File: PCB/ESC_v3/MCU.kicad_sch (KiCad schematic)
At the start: 48 parts, among them J10 Conn_01x01_Pin, J3 Conn_01x01_Pin, J4 Conn_01x01_Pin, J5 Conn_01x01_Pin, J6 Conn_01x01_Pin, J7 Conn_01x01_Pin, J8 Conn_01x01_Pin, J9 Conn_01x01_Pin, U3 STM32G474CETx, Y2 24MHz

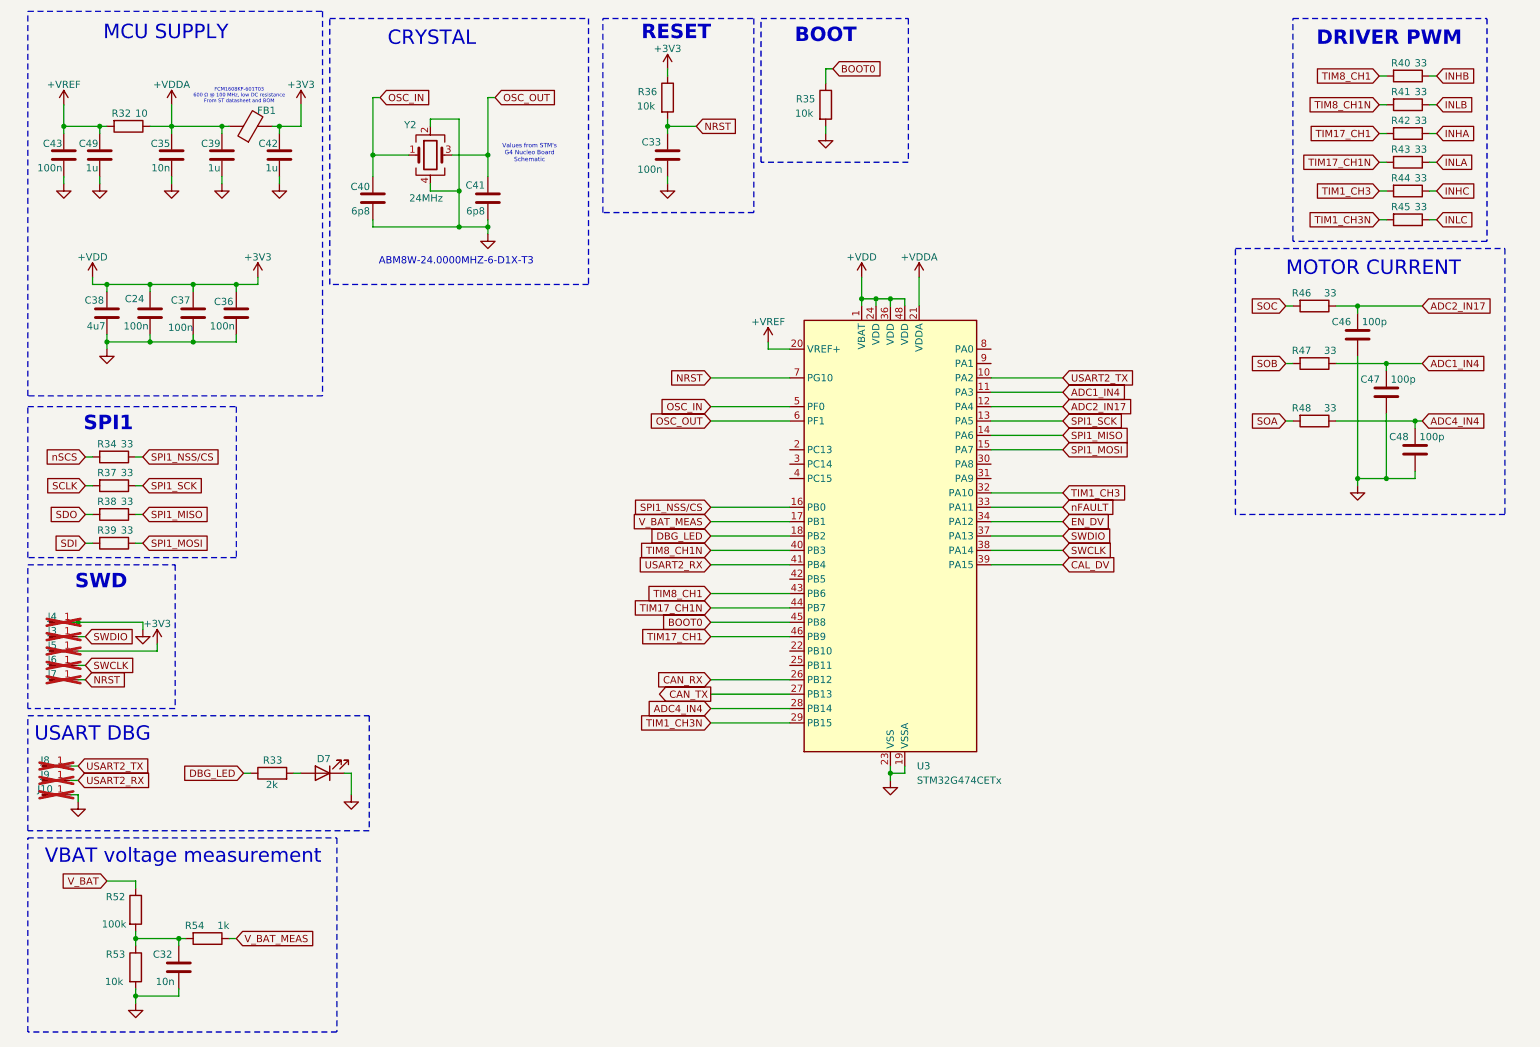
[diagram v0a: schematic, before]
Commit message: Layout update
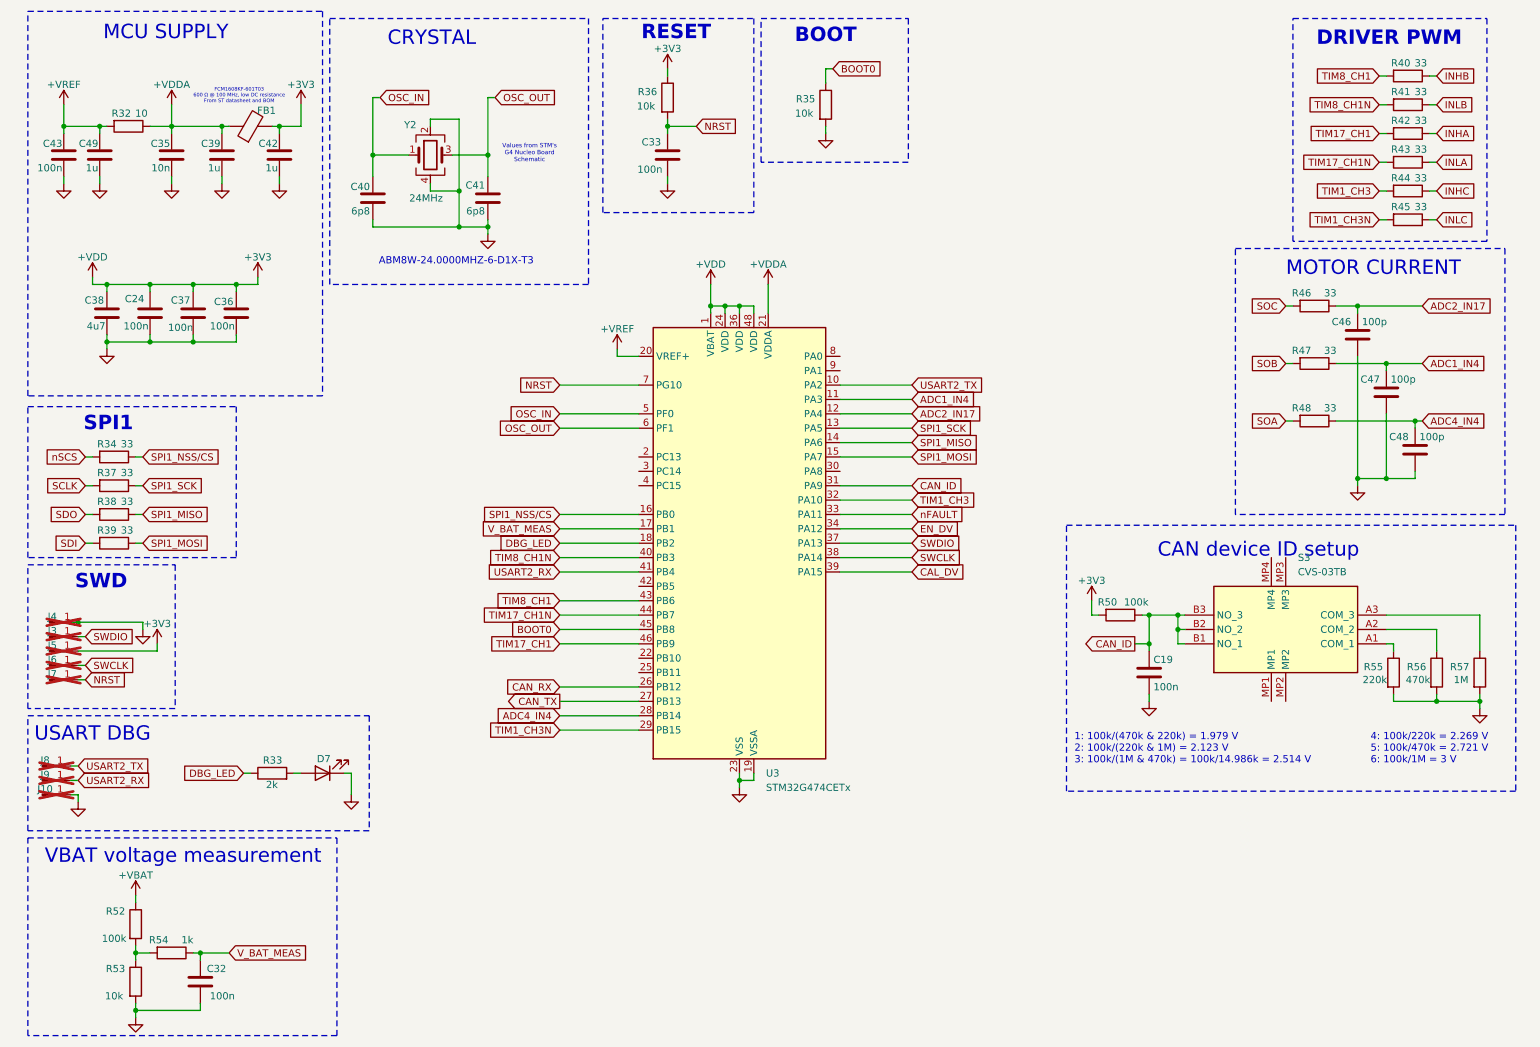
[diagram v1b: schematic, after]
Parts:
- added C19: 100n, Capacitor_SMD:C_0402_1005Metric, symbol Device:C
- added R50: 100k, Resistor_SMD:R_0603_1608Metric, symbol Device:R
- added R55: 220k, Resistor_SMD:R_0603_1608Metric, symbol Device:R
- added R56: 470k, Resistor_SMD:R_0603_1608Metric, symbol Device:R
- added R57: 1M, Resistor_SMD:R_0603_1608Metric, symbol Device:R
- added S3: CVS-03TB, CVS03TB, symbol SamacSys_Parts:CVS-03TB
- C32: value 10n -> 100n
- C37: footprint Capacitor_SMD:C_0805_2012Metric -> Capacitor_SMD:C_0603_1608Metric
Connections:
- net +3V3: now also R50.2
- net GND: now also C19.2, R55.2, R56.2, R57.2
- net V_BAT_MEAS: now also C32.1
- net at R52.2, R53.1, R54.2: no longer C32.1
- net CAN_ID: now reaches U3.31 (PA9)
- net CAN_ID: now also C19.1, R50.1, S3.B1 (NO_1), S3.B2 (NO_2), S3.B3 (NO_3)
- net V_BAT renamed +VBAT
- new net: R56.1, S3.A2 (COM_2)
- new net: R57.1, S3.A3 (COM_3)
- new net: R55.1, S3.A1 (COM_1)
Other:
- note added: "1: 100k/(470k & 220k) = 1.979 V 2: 100k/(220k & 1M) = 2.123 V 3: 100k/(1M & 470k) = 100k/14.986k = 2.514 V"
- note added: "4: 100k/220k = 2.269 V 5: 100k/470k = 2.721 V 6: 100k/1M = 3 V"
- note added: "CAN device ID setup"
- moved on the sheet: C32, R52, R53, R54, U3
